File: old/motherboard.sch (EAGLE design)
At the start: 34 parts

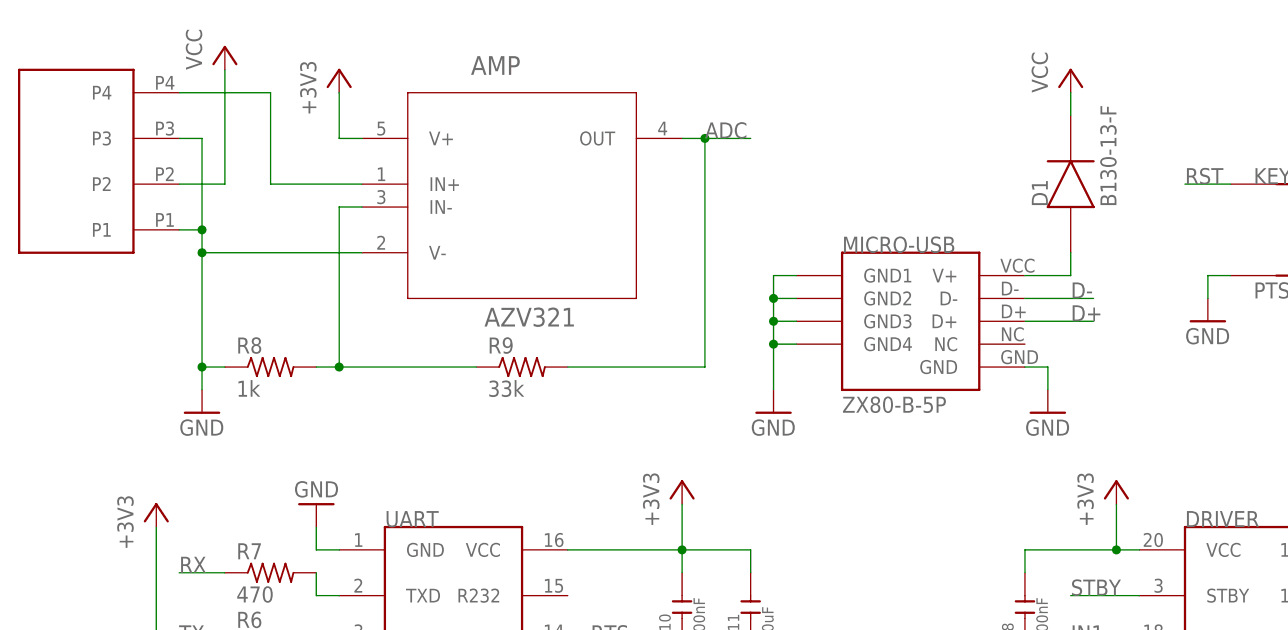
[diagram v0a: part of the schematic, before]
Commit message: started work on revised board
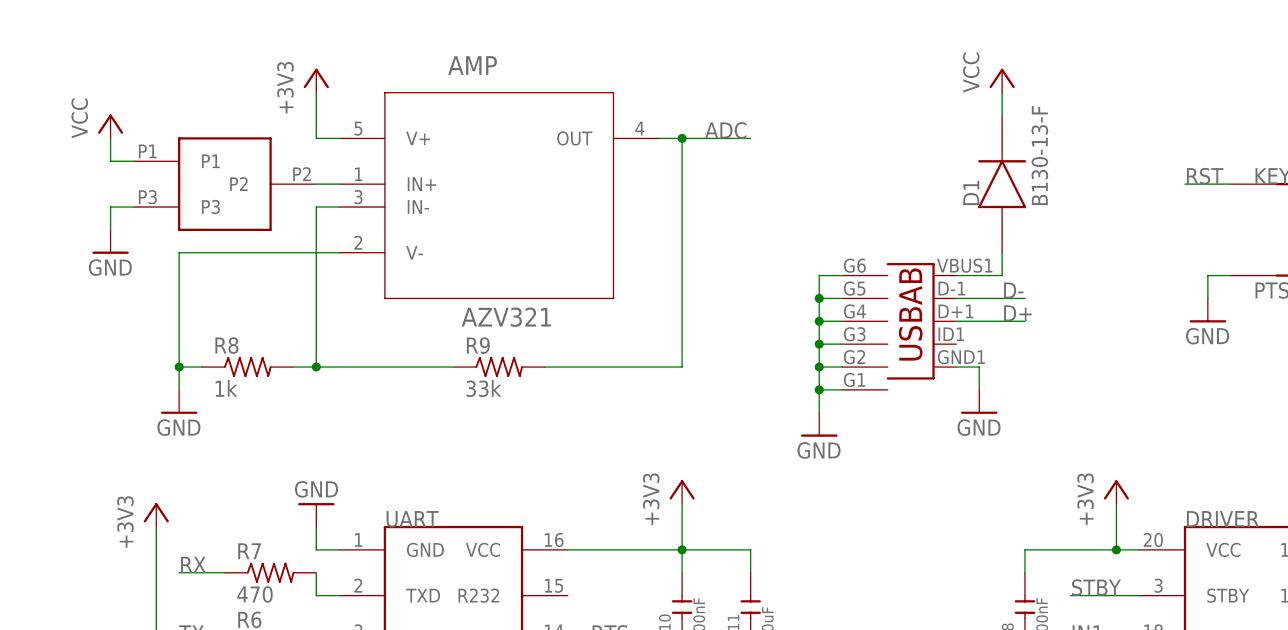
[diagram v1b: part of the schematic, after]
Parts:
- removed MICRO-USB: ZX80-B-5P, CUSTOM:USB_VERT
- removed U$1: BOURNS_4PIN, CUSTOM:BOURNS_4PIN
- added CONN: AVX_CONN, CUSTOM:AVX_CONN
- added USB: (no value), MicroUSB:USB""
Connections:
- net D+: now also USB.D+; no longer MICRO-USB.D+
- net D-: now also USB.D-; no longer MICRO-USB.D-
- net GND: now also CONN.P3, USB.G1, USB.G2, USB.G3, USB.G4, USB.G5, USB.G6, USB.GND; no longer MICRO-USB.GND, MICRO-USB.GND1, MICRO-USB.GND2, MICRO-USB.GND3, MICRO-USB.GND4, U$1.P1, U$1.P3
- net N$3: now also USB.VBUS; no longer MICRO-USB.V+
- net N$5: now also CONN.P2; no longer U$1.P4
- net VCC: now also CONN.P1; no longer U$1.P2
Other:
- moved on the sheet: AMP, D1, R8, R9
